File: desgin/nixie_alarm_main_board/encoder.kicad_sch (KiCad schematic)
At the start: 10 parts

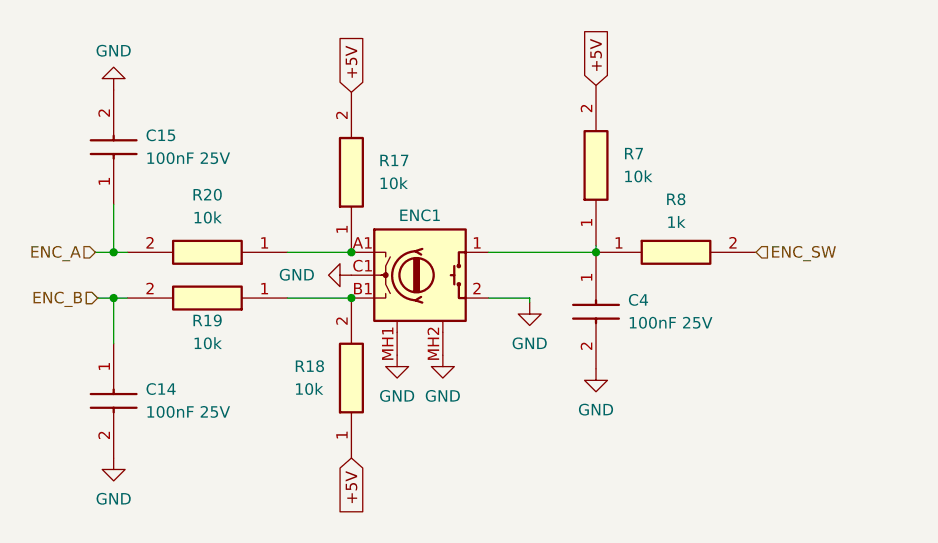
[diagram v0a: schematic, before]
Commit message: board v2
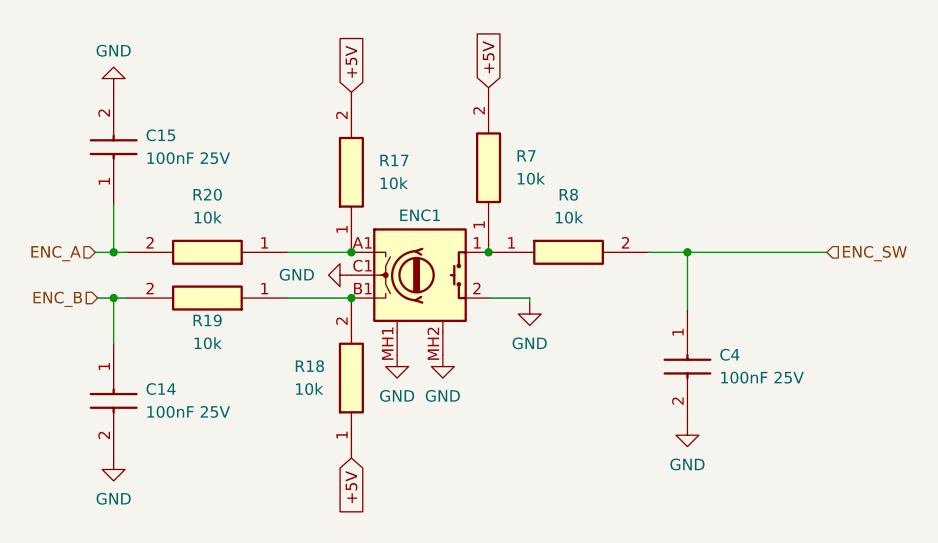
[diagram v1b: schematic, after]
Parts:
- R8: value 1k -> 10k
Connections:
- net ENC_SW: now also C4.1
- net at ENC1.1, R7.1, R8.1: no longer C4.1
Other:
- moved on the sheet: C4, R7, R8
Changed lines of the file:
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@@
 	(paper "A4")
+	(junction
+		(at 188.468 88.9)
+		(diameter 0)
+		(color 0 0 0 0)
+	)
 	(junction
 		(at 151.13 88.9)
@@
 	)
 	(junction
-		(at 178.308 88.9)
-		(diameter 0)
-		(color 0 0 0 0)
-	)
-	(junction
 		(at 124.714 93.98)
 		(diameter 0)
 		(color 0 0 0 0)
 	)
+	(junction
+		(at 166.37 88.9)
+		(diameter 0)
+		(color 0 0 0 0)
+	)
 	(wire
 		(pts
@@
 	(wire
 		(pts
-			(xy 178.308 88.9) (xy 178.308 89.154)
+			(xy 144.018 88.9) (xy 151.13 88.9)
 		)
 		(stroke
@@
 	(wire
 		(pts
-			(xy 144.018 88.9) (xy 151.13 88.9)
+			(xy 124.714 83.566) (xy 124.714 88.9)
 		)
 		(stroke
@@
 	(wire
 		(pts
-			(xy 124.714 83.566) (xy 124.714 88.9)
+			(xy 166.37 88.392) (xy 166.37 88.9)
 		)
 		(stroke
@@
 	(wire
 		(pts
-			(xy 178.308 88.138) (xy 178.308 88.9)
+			(xy 124.714 93.98) (xy 126.238 93.98)
 		)
 		(stroke
@@
 	(wire
 		(pts
-			(xy 124.714 93.98) (xy 126.238 93.98)
+			(xy 124.714 88.9) (xy 126.238 88.9)
 		)
 		(stroke
@@
 	(wire
 		(pts
-			(xy 124.714 88.9) (xy 126.238 88.9)
+			(xy 188.468 88.9) (xy 184.15 88.9)
 		)
 		(stroke
@@
 	(wire
 		(pts
-			(xy 166.37 88.9) (xy 178.308 88.9)
+			(xy 188.468 95.25) (xy 188.468 88.9)
 		)
 		(stroke
@@
 	(wire
 		(pts
-			(xy 170.942 93.98) (xy 170.942 94.488)
+			(xy 203.962 88.9) (xy 188.468 88.9)
 		)
 		(stroke
@@
 	(wire
 		(pts
-			(xy 122.682 88.9) (xy 124.714 88.9)
+			(xy 170.942 93.98) (xy 170.942 94.488)
 		)
 		(stroke
@@
 	(wire
 		(pts
-			(xy 144.018 93.98) (xy 151.13 93.98)
+			(xy 122.682 88.9) (xy 124.714 88.9)
 		)
 		(stroke
@@
 		)
 	)
+	(wire
+		(pts
+			(xy 144.018 93.98) (xy 151.13 93.98)
+		)
+		(stroke
+			(width 0)
+			(type default)
+		)
+	)
 	(global_label "+5V"
 		(shape input)
-		(at 178.308 70.358 90)
+		(at 166.37 70.612 90)
 		(fields_autoplaced yes)
 		(effects
@@
 		)
 		(property "Intersheetrefs" "${INTERSHEET_REFS}"
-			(at 178.308 63.5023 90)
+			(at 166.37 63.7563 90)
 			(effects
 				(font
@@
 	(hierarchical_label "ENC_SW"
 		(shape input)
-		(at 196.088 88.9 0)
+		(at 203.962 88.9 0)
 		(fields_autoplaced yes)
 		(effects
@@
 	(symbol
 		(lib_id "SamacSys_Parts:ERJ-UP6D5101V")
-		(at 178.308 88.138 90)
+		(at 166.37 88.392 90)
 		(unit 1)
 		(exclude_from_sim no)
@@
 		(fields_autoplaced yes)
 		(property "Reference" "R7"
-			(at 181.356 77.9779 90)
+			(at 169.418 78.2319 90)
 			(effects
 				(font
@@
 		)
 		(property "Value" "10k"
-			(at 181.356 80.5179 90)
+			(at 169.418 80.7719 90)
 			(effects
 				(font
@@
 		)
 		(property "Footprint" "Resistor_SMD:R_0805_2012Metric_Pad1.20x1.40mm_HandSolder"
-			(at 274.498 74.168 0)
+			(at 262.56 74.422 0)
 			(effects
 				(font
@@
 		)
 		(property "Datasheet" "https://industrial.panasonic.com/cdbs/www-data/pdf/RDP0000/AOA0000C337.pdf"
-			(at 374.498 74.168 0)
+			(at 362.56 74.422 0)
 			(effects
 				(font
@@
 		)
 		(property "Description" "Anti-Sulfurated Thick Film Chip Resistors/ Anti-Surge Type, Power Rating (W): 0.5, Chip Size (LxW(EIA)) (mm): 2.0 x 1.25 (EIA:0805), Resistance Values (?): 5100, Resistance Tolerance (%): 0.5, T.C.R (?102/K): ?100"
-			(at 178.308 88.138 0)
+			(at 166.37 88.392 0)
 			(effects
 				(font
@@
 		)
 		(property "Height" "0.7"
-			(at 574.498 74.168 0)
+			(at 562.56 74.422 0)
 			(effects
 				(font
@@
 		)
 		(property "Mouser Part Number" "667-ERJ-UP6D5101V"
-			(at 674.498 74.168 0)
+			(at 662.56 74.422 0)
 			(effects
 				(font
@@
 		)
 		(property "Mouser Price/Stock" "https://www.mouser.co.uk/ProductDetail/Panasonic/ERJ-UP6D5101V?qs=ZcfC38r4Pouz7%2FLHthUDHQ%3D%3D"
-			(at 774.498 74.168 0)
+			(at 762.56 74.422 0)
 			(effects
 				(font
@@
 		)
 		(property "Manufacturer_Name" "Panasonic"
-			(at 874.498 74.168 0)
+			(at 862.56 74.422 0)
 			(effects
 				(font
@@
 		)
 		(property "Manufacturer_Part_Number" "ERJ-UP6D5101V"
-			(at 974.498 74.168 0)
+			(at 962.56 74.422 0)
 			(effects
 				(font
@@
 	(symbol
 		(lib_id "SamacSys_Parts:ERJ-UP6D5101V")
-		(at 178.308 88.9 0)
+		(at 166.37 88.9 0)
 		(unit 1)
 		(exclude_from_sim no)
@@
 		(fields_autoplaced yes)
 		(property "Reference" "R8"
-			(at 187.198 83.058 0)
-			(effects
-				(font
-					(size 1.27 1.27)
-				)
-			)
-		)
-		(property "Value" "1k"
-			(at 187.198 85.598 0)
+			(at 175.26 82.55 0)
+			(effects
+				(font
+					(size 1.27 1.27)
+				)
+			)
+		)
+		(property "Value" "10k"
+			(at 175.26 85.09 0)
 			(effects
 				(font
@@
 		)
 		(property "Footprint" "Resistor_SMD:R_0805_2012Metric_Pad1.20x1.40mm_HandSolder"
-			(at 192.278 185.09 0)
+			(at 180.34 185.09 0)
 			(effects
 				(font
@@
 		)
 		(property "Datasheet" "https://industrial.panasonic.com/cdbs/www-data/pdf/RDP0000/AOA0000C337.pdf"
-			(at 192.278 285.09 0)
+			(at 180.34 285.09 0)
 			(effects
 				(font
@@
 		)
 		(property "Description" "Anti-Sulfurated Thick Film Chip Resistors/ Anti-Surge Type, Power Rating (W): 0.5, Chip Size (LxW(EIA)) (mm): 2.0 x 1.25 (EIA:0805), Resistance Values (?): 5100, Resistance Tolerance (%): 0.5, T.C.R (?102/K): ?100"
-			(at 178.308 88.9 0)
+			(at 166.37 88.9 0)
 			(effects
 				(font
@@
 		)
 		(property "Height" "0.7"
-			(at 192.278 485.09 0)
+			(at 180.34 485.09 0)
 			(effects
 				(font
@@
 		)
 		(property "Mouser Part Number" "667-ERJ-UP6D5101V"
-			(at 192.278 585.09 0)
+			(at 180.34 585.09 0)
 			(effects
 				(font
@@
 		)
 		(property "Mouser Price/Stock" "https://www.mouser.co.uk/ProductDetail/Panasonic/ERJ-UP6D5101V?qs=ZcfC38r4Pouz7%2FLHthUDHQ%3D%3D"
-			(at 192.278 685.09 0)
+			(at 180.34 685.09 0)
 			(effects
 				(font
@@
 		)
 		(property "Manufacturer_Name" "Panasonic"
-			(at 192.278 785.09 0)
+			(at 180.34 785.09 0)
 			(effects
 				(font
@@
 		)
 		(property "Manufacturer_Part_Number" "ERJ-UP6D5101V"
-			(at 192.278 885.09 0)
+			(at 180.34 885.09 0)
 			(effects
 				(font
@@
 	(symbol
 		(lib_id "power:GND")
-		(at 178.308 101.854 0)
+		(at 188.468 107.95 0)
 		(unit 1)
 		(exclude_from_sim no)
@@
 		(fields_autoplaced yes)
 		(property "Reference" "#PWR08"
-			(at 178.308 108.204 0)
+			(at 188.468 114.3 0)
 			(effects
 				(font
@@
 		)
 		(property "Value" "GND"
-			(at 178.308 106.426 0)
+			(at 188.468 112.522 0)
 			(effects
 				(font
@@
 		)
 		(property "Footprint" ""
-			(at 178.308 101.854 0)
+			(at 188.468 107.95 0)
 			(effects
 				(font
@@
 		)
 		(property "Datasheet" ""
-			(at 178.308 101.854 0)
+			(at 188.468 107.95 0)
 			(effects
 				(font
@@
 		)
 		(property "Description" "Power symbol creates a global label with name \"GND\" , ground"
-			(at 178.308 101.854 0)
+			(at 188.468 107.95 0)
 			(effects
 				(font
@@
 	(symbol
 		(lib_id "SamacSys_Parts:GRM033R71E101KA01J")
-		(at 178.308 89.154 270)
+		(at 188.468 95.25 270)
 		(unit 1)
 		(exclude_from_sim no)
@@
 		(fields_autoplaced yes)
 		(property "Reference" "C4"
-			(at 181.864 94.2339 90)
+			(at 192.024 100.3299 90)
 			(effects
 				(font
@@
 		)
 		(property "Value" "100nF 25V"
-			(at 181.864 96.7739 90)
+			(at 192.024 102.8699 90)
 			(effects
 				(font
@@
 		)
 		(property "Footprint" "Capacitor_SMD:C_0805_2012Metric_Pad1.18x1.45mm_HandSolder"
-			(at 82.118 98.044 0)
+			(at 92.278 104.14 0)
 			(effects
 				(font
@@
 		)
 		(property "Datasheet" "https://search.murata.co.jp/Ceramy/image/img/A01X/G101/ENG/GRM033R71E101KA01-01A.pdf"
-			(at -17.882 98.044 0)
+			(at -7.722 104.14 0)
 			(effects
 				(font
@@
 		)
 		(property "Description" "Multilayer Ceramic Capacitors MLCC - SMD/SMT 100pF 25 volts 10%"
-			(at 178.308 89.154 0)
+			(at 188.468 95.25 0)
 			(effects
 				(font
@@
 		)
 		(property "Height" "0.5"
-			(at -217.882 98.044 0)
+			(at -207.722 104.14 0)
 			(effects
 				(font
@@
 		)
 		(property "Mouser Part Number" "81-GRM033R71E101KA1J"
-			(at -317.882 98.044 0)
+			(at -307.722 104.14 0)
 			(effects
 				(font
@@
 		)
 		(property "Mouser Price/Stock" "https://www.mouser.co.uk/ProductDetail/Murata-Electronics/GRM033R71E101KA01J?qs=563MOeNa05Lmru4oTW10Jw%3D%3D"
-			(at -417.882 98.044 0)
+			(at -407.722 104.14 0)
 			(effects
 				(font
@@
 		)
 		(property "Manufacturer_Name" "Murata Electronics"
-			(at -517.882 98.044 0)
+			(at -507.722 104.14 0)
 			(effects
 				(font
@@
 		)
 		(property "Manufacturer_Part_Number" "GRM033R71E101KA01J"
-			(at -617.882 98.044 0)
-			(effects
-				(font
+			(at -607.722 104.14 0)
+			(effects
+				(font
